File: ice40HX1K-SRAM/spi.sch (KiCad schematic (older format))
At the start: 9 parts, among them J2 Conn_02x05_Odd_Even, U5 AT25SF081-SSHD-X

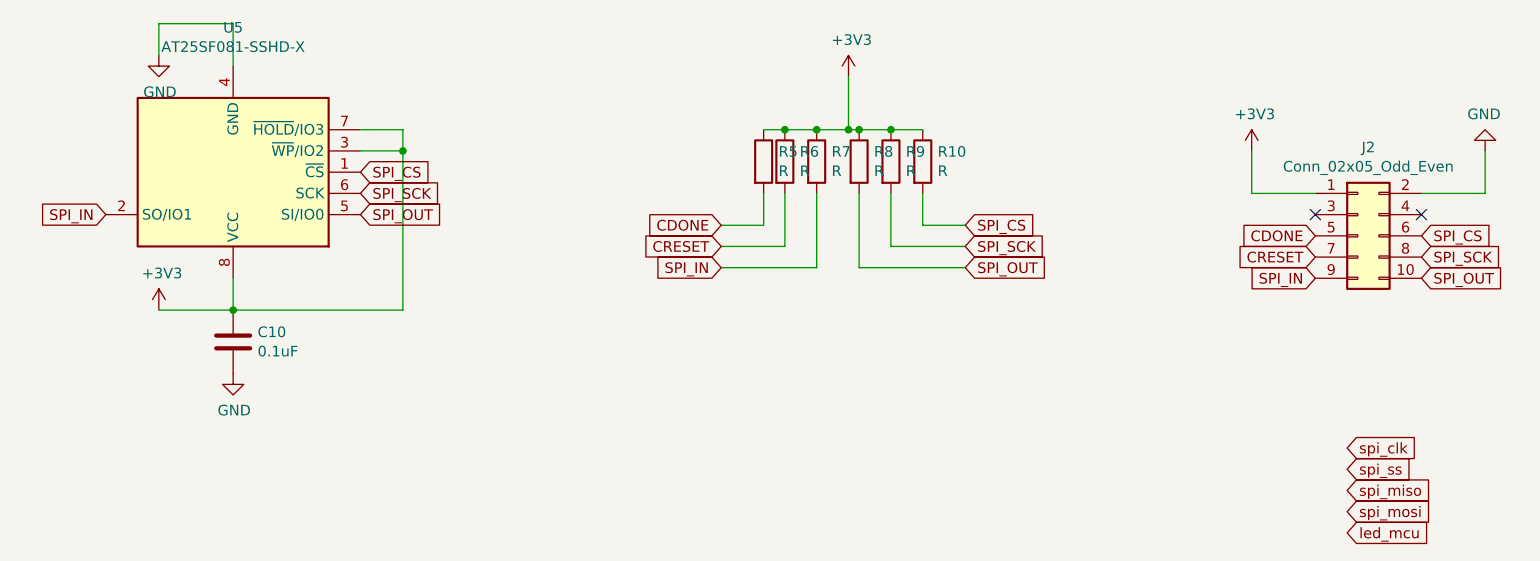
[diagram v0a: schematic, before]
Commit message: wiring FPGA
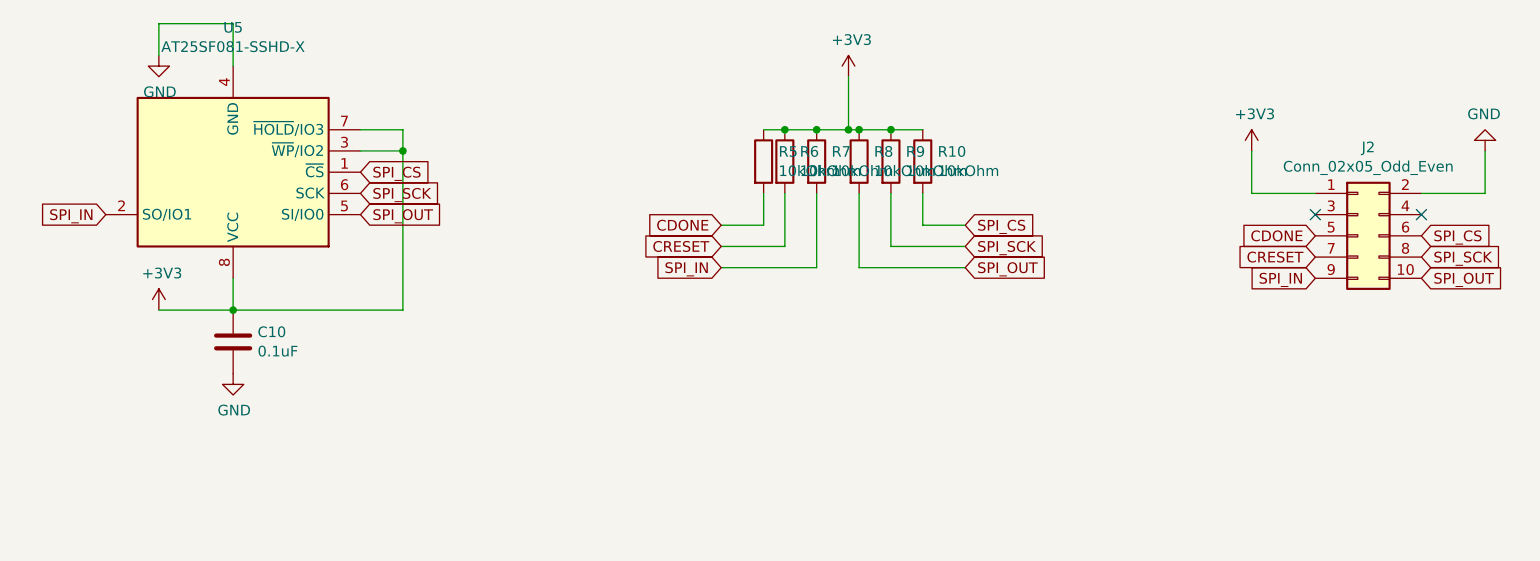
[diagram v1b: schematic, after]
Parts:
- C10: footprint Capacitor_SMD:C_0805_2012Metric -> Capacitor_SMD:C_0402_1005Metric
- R10, R5, R6, R7, R8, R9: value R -> 10kOhm; footprint Resistor_SMD:R_1206_3216Metric -> Resistor_SMD:R_0402_1005Metric
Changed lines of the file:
@@
 F 0 "C10" H 2415 2746 50  0000 L CNN
 F 1 "0.1uF" H 2415 2655 50  0000 L CNN
-F 2 "Capacitor_SMD:C_0805_2012Metric" H 2338 2550 50  0001 C CNN
+F 2 "Capacitor_SMD:C_0402_1005Metric" H 2338 2550 50  0001 C CNN
 F 3 "~" H 2300 2700 50  0001 C CNN
 	1    2300 2700
@@
 AR Path="/5E5F2441/5E62B581" Ref="R7"  Part="1"
 F 0 "R7" H 5120 1896 50  0000 L CNN
-F 1 "R" H 5120 1805 50  0000 L CNN
-F 2 "Resistor_SMD:R_1206_3216Metric" V 4980 1850 50  0001 C CNN
+F 1 "10kOhm" H 5120 1805 50  0000 L CNN
+F 2 "Resistor_SMD:R_0402_1005Metric" V 4980 1850 50  0001 C CNN
 F 3 "~" H 5050 1850 50  0001 C CNN
 	1    5050 1850
@@
 AR Path="/5E5F2441/5E62B587" Ref="R8"  Part="1"
 F 0 "R8" H 5320 1896 50  0000 L CNN
-F 1 "R" H 5320 1805 50  0000 L CNN
-F 2 "Resistor_SMD:R_1206_3216Metric" V 5180 1850 50  0001 C CNN
+F 1 "10kOhm" H 5320 1805 50  0000 L CNN
+F 2 "Resistor_SMD:R_0402_1005Metric" V 5180 1850 50  0001 C CNN
 F 3 "~" H 5250 1850 50  0001 C CNN
 	1    5250 1850
@@
 AR Path="/5E5F2441/5E62B58D" Ref="R9"  Part="1"
 F 0 "R9" H 5470 1896 50  0000 L CNN
-F 1 "R" H 5470 1805 50  0000 L CNN
-F 2 "Resistor_SMD:R_1206_3216Metric" V 5330 1850 50  0001 C CNN
+F 1 "10kOhm" H 5470 1805 50  0000 L CNN
+F 2 "Resistor_SMD:R_0402_1005Metric" V 5330 1850 50  0001 C CNN
 F 3 "~" H 5400 1850 50  0001 C CNN
 	1    5400 1850
@@
 AR Path="/5E5F2441/5E62B593" Ref="R10"  Part="1"
 F 0 "R10" H 5620 1896 50  0000 L CNN
-F 1 "R" H 5620 1805 50  0000 L CNN
-F 2 "Resistor_SMD:R_1206_3216Metric" V 5480 1850 50  0001 C CNN
+F 1 "10kOhm" H 5620 1805 50  0000 L CNN
+F 2 "Resistor_SMD:R_0402_1005Metric" V 5480 1850 50  0001 C CNN
 F 3 "~" H 5550 1850 50  0001 C CNN
 	1    5550 1850
@@
 AR Path="/5E5F2441/5E62B599" Ref="R5"  Part="1"
 F 0 "R5" H 4870 1896 50  0000 L CNN
-F 1 "R" H 4870 1805 50  0000 L CNN
-F 2 "Resistor_SMD:R_1206_3216Metric" V 4730 1850 50  0001 C CNN
+F 1 "10kOhm" H 4870 1805 50  0000 L CNN
+F 2 "Resistor_SMD:R_0402_1005Metric" V 4730 1850 50  0001 C CNN
 F 3 "~" H 4800 1850 50  0001 C CNN
 	1    4800 1850
@@
 AR Path="/5E5F2441/5E62B59F" Ref="R6"  Part="1"
 F 0 "R6" H 4970 1896 50  0000 L CNN
-F 1 "R" H 4970 1805 50  0000 L CNN
-F 2 "Resistor_SMD:R_1206_3216Metric" V 4830 1850 50  0001 C CNN
+F 1 "10kOhm" H 4970 1805 50  0000 L CNN
+F 2 "Resistor_SMD:R_0402_1005Metric" V 4830 1850 50  0001 C CNN
 F 3 "~" H 4900 1850 50  0001 C CNN
 	1    4900 1850
@@
 NoConn ~ 7900 2100
 NoConn ~ 7400 2100
-Text GLabel 7550 3200 2    50   Input ~ 0
-spi_clk
-Text GLabel 7550 3300 2    50   Input ~ 0
-spi_ss
-Text GLabel 7550 3400 2    50   Input ~ 0
-spi_miso
-Text GLabel 7550 3500 2    50   Input ~ 0
-spi_mosi
-Text GLabel 7550 3600 2    50   Input ~ 0
-led_mcu
 $EndSCHEMATC
